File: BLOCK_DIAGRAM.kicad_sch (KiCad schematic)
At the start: 0 parts

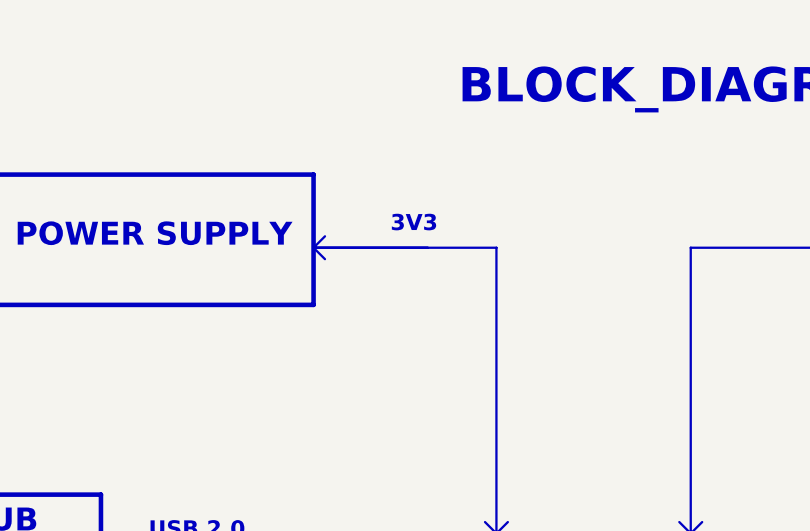
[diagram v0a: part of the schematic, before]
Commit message: new
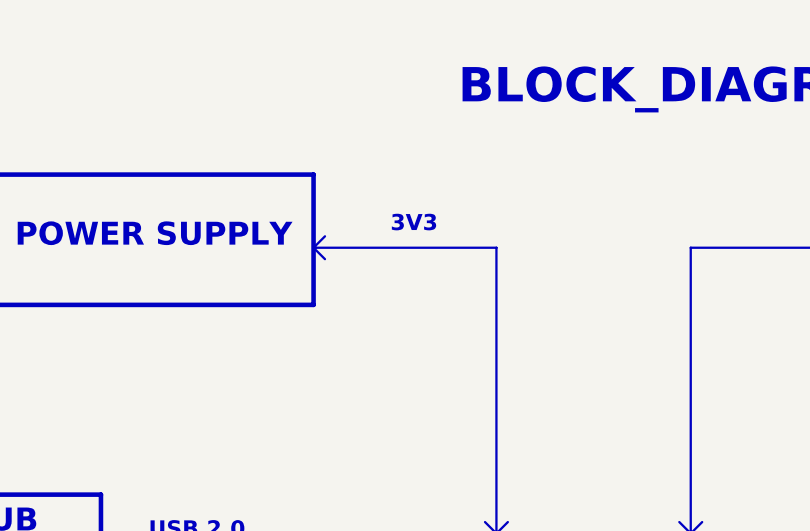
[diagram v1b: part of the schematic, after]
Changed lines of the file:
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@@
+	(polyline
+		(pts
+			(xy 124.46 38.1) (xy 104.14 38.1)
+		)
+		(stroke
+			(width 0.254)
+			(type default)
+			(color 0 0 194 1)
+		)
+	)
 	(polyline
 		(pts
@@
 	(polyline
 		(pts
-			(xy 104.14 38.1) (xy 124.46 38.1)
-		)
-		(stroke
-			(width 0.254)
-			(type default)
-			(color 0 0 194 1)
-		)
-	)
-	(polyline
-		(pts
 			(xy 102.87 96.52) (xy 104.14 95.25)
 		)
@@
 		)
 		(stroke
-			(width 0.254)
-			(type default)
-			(color 0 0 0 1)
-		)
-	)
-	(polyline
-		(pts
-			(xy 104.14 38.1) (xy 116.84 38.1)
-		)
-		(stroke
